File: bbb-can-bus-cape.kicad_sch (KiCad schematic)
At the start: 5 parts, among them P1 DG301-5.0-03P-12-00A(H), P2 DG301-5.0-03P-12-00A(H), P7 DG301-5.0-03P-12-00A(H), P8 BeagleBone_Black_Header, P9 BeagleBone_Black_Header

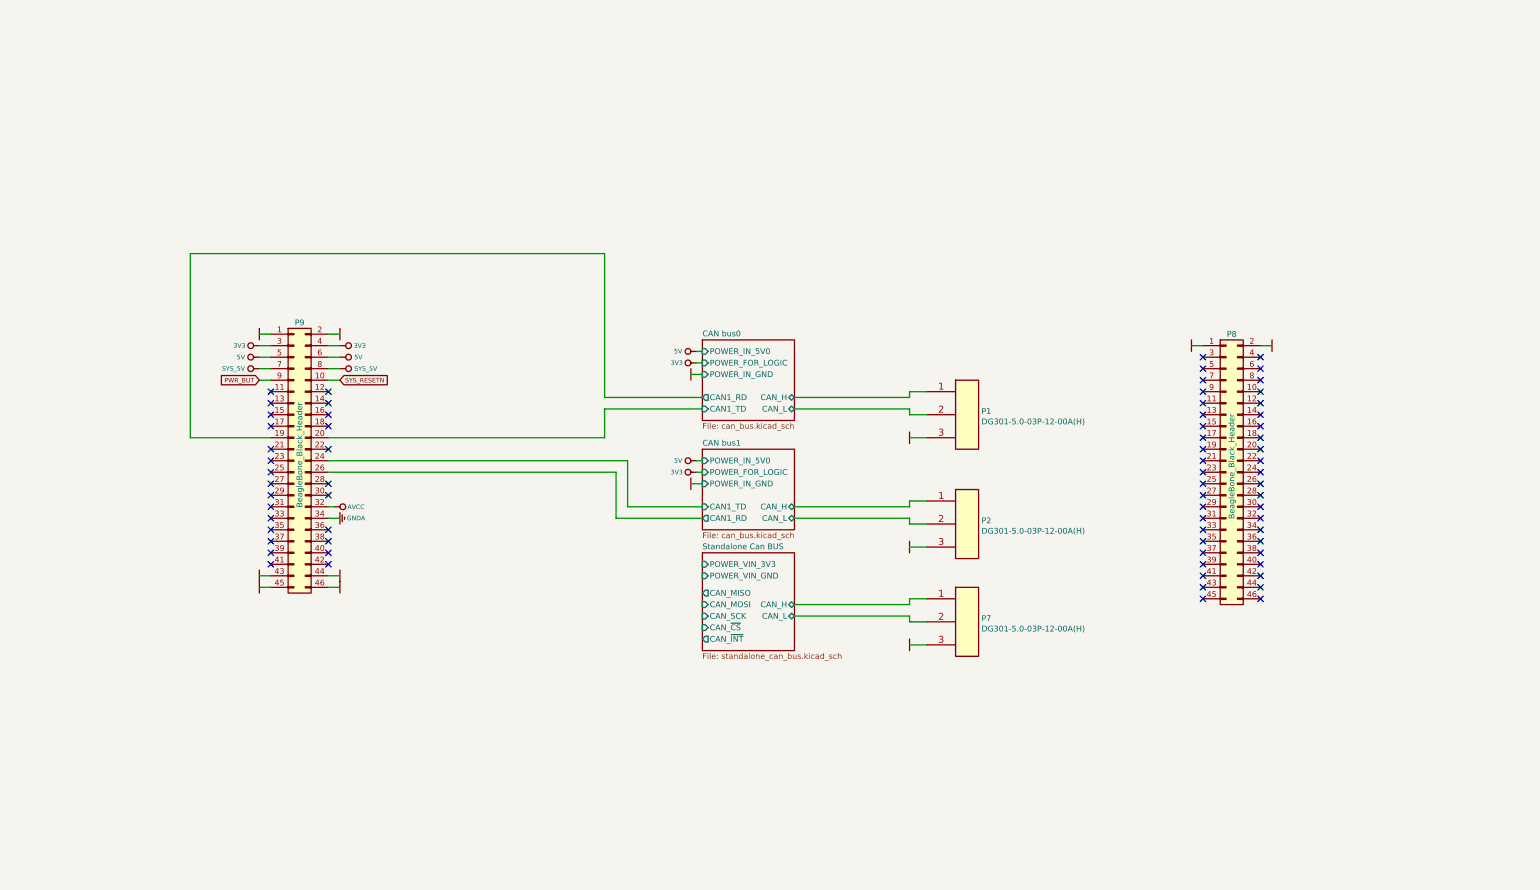
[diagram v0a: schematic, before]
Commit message: Schematic checked
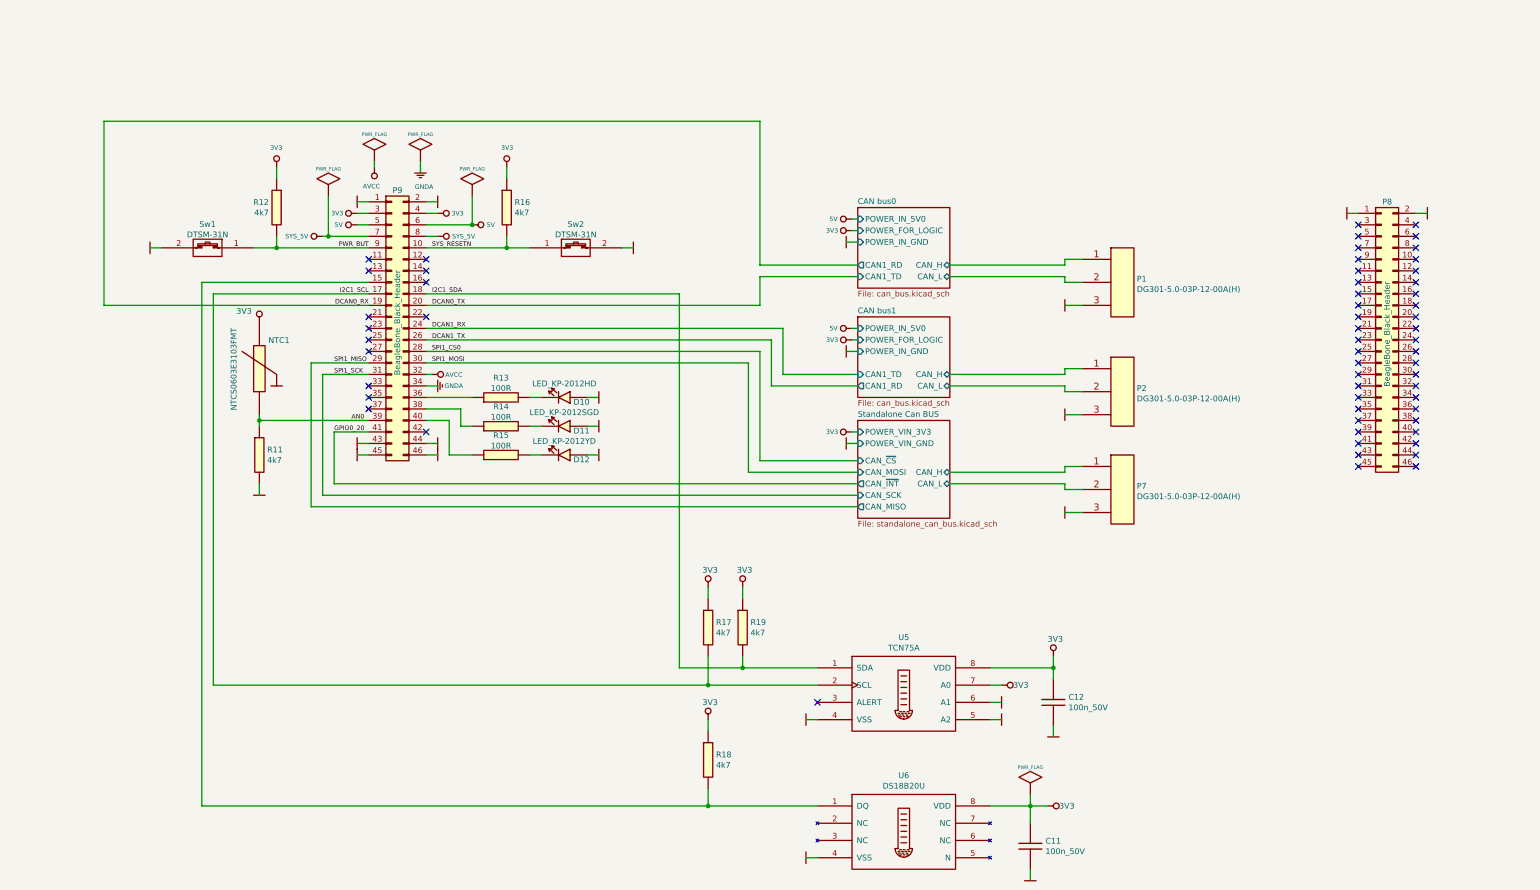
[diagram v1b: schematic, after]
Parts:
- added C11, C12: 100n_50V, Capacitors_Smd_0603:100nF_0603, symbol Capacitors_Smd0603:100n
- added D10: LED_KP-2012HD, Diodes:LED_KP-2012HD_SM0805, symbol Diodes:LED_KP-2012HD
- added D11: LED_KP-2012SGD, Diodes:LED_KP-2012SGD_SM0805, symbol Diodes:LED_KP-2012SGD
- added D12: LED_KP-2012YD, Diodes:LED_KP-2012YD_SM0805, symbol Diodes:LED_KP-2012YD
- added NTC1: NTCS0603E3103FMT, NTC_Thermistors:NTCS0603E3103FMT, symbol NTC_Thermistors:NTCS0603E3103FMT
- added R11, R12, R16, R17, R18, R19: 4k7, Resistor_Smd_0603:4k7_0603, symbol Resistors_Smd0603:4k7
- added R13, R14, R15: 100R, Resistor_Smd_0603:100R_0603, symbol Resistors_Smd0603:100R
- added Sw1, Sw2: DTSM-31N, Microswitches:DTSM-31N_SMD, symbol Microswitches:DTSM-31N
- added U5: TCN75A, Temperature_Sensors:TCN75A_SOIC8, symbol Temperature_Sensors:TCN75A
- added U6: DS18B20U, Temperature_Sensors:DS18B20U_MSOP-8_3x3mm_P0.65mm, symbol Temperature_Sensors:DS18B20U
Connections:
- net 3V3: now also C11.1, C12.1, NTC1.2, R12.1, R16.1, R17.1, R18.1, R19.1, U5.7 (A0), U5.8 (VDD), U6.8 (VDD)
- net GND: now also C11.2, C12.2, D10.1 (A), D11.1 (A), D12.1 (A), R11.2, Sw1.2, Sw2.2, U5.4 (VSS), U5.5 (A2), U5.6 (A1), U6.4 (VSS)
- net PWR_BUT: now also R12.2, Sw1.1
- net SYS_RESETN: now also R16.2, Sw2.1
- net at P9.15 (Pin_15): now also R18.2, U6.1 (DQ)
- net I2C1_SCL: now reaches P9.17 (Pin_17)
- net I2C1_SCL: now also R17.2, U5.2 (SCL)
- net I2C1_SDA: now reaches P9.18 (Pin_18)
- net I2C1_SDA: now also R19.2, U5.1 (SDA)
- net SPI1_CS0: now reaches P9.28 (Pin_28)
- net SPI1_MISO: now reaches P9.29 (Pin_29)
- net SPI1_MOSI: now reaches P9.30 (Pin_30)
- net SPI1_SCK: now reaches P9.31 (Pin_31)
- net at P9.36 (Pin_36): now also R13.1
- net at P9.38 (Pin_38): now also R14.1
- net AN0: now reaches P9.39 (Pin_39)
- net AN0: now also NTC1.1, R11.1
- net at P9.40 (Pin_40): now also R15.1
- net GPIO0_20: now reaches P9.41 (Pin_41)
- net CAN bus0/CAN1_RD renamed DCAN0_RX
- net CAN bus0/CAN1_TD renamed DCAN0_TX
- net CAN bus1/CAN1_RD renamed DCAN1_TX
- net CAN bus1/CAN1_TD renamed DCAN1_RX
- new net: D11.2 (K), R14.2
- new net: D10.2 (K), R13.2
- new net: D12.2 (K), R15.2
- no-connect marks 70 -> 59
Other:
- moved on the sheet: P1, P2, P7, P8, P9

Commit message: Finalized project
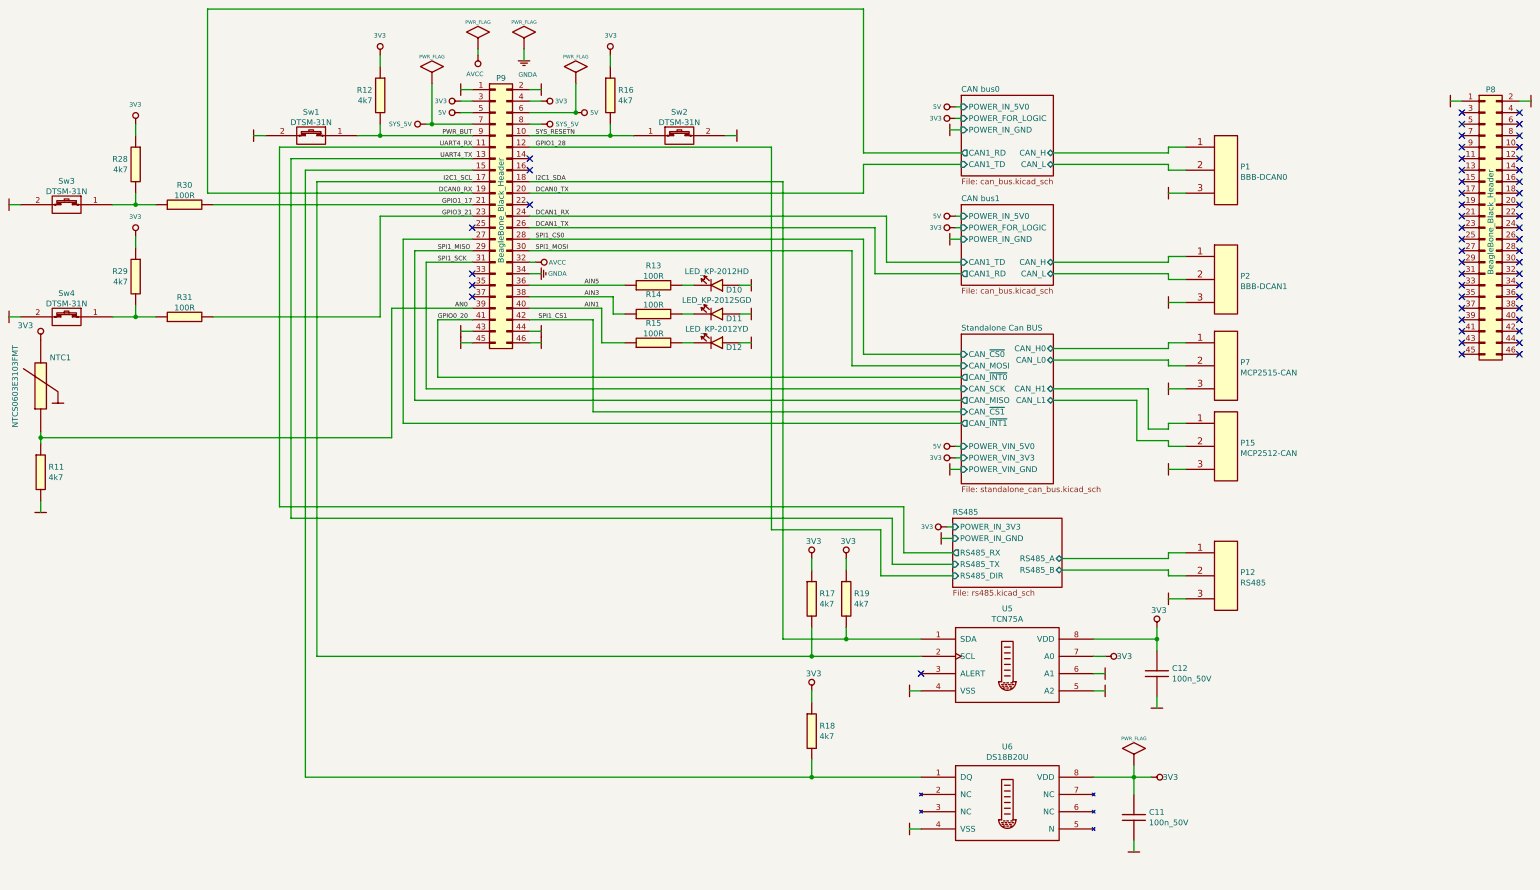
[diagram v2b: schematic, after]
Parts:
- added P12: RS485, Discrete_Connectors:DG301-5.0-03P-12-00A(H), symbol Discrete_Connectors:DG301-5.0-03P-12-00A(H)
- added P15: MCP2512-CAN, Discrete_Connectors:DG301-5.0-03P-12-00A(H), symbol Discrete_Connectors:DG301-5.0-03P-12-00A(H)
- added R28, R29: 4k7, Resistor_Smd_0603:4k7_0603, symbol Resistors_Smd0603:4k7
- added R30, R31: 100R, Resistor_Smd_0603:100R_0603, symbol Resistors_Smd0603:100R
- added Sw3, Sw4: DTSM-31N, Microswitches:DTSM-31N_SMD, symbol Microswitches:DTSM-31N
- P1: value DG301-5.0-03P-12-00A(H) -> BBB-DCAN0
- P2: value DG301-5.0-03P-12-00A(H) -> BBB-DCAN1
- P7: value DG301-5.0-03P-12-00A(H) -> MCP2515-CAN
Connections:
- net 3V3: now also R28.1, R29.1
- net GND: now also P12.3, P15.3, Sw3.2, Sw4.2
- net UART4_RX: now reaches P9.11 (Pin_11)
- net GPIO1_28: now reaches P9.12 (Pin_12)
- net UART4_TX: now reaches P9.13 (Pin_13)
- net GPIO1_17: now reaches P9.21 (Pin_21)
- net GPIO1_17: now also R30.2
- net GPIO3_21: now reaches P9.23 (Pin_23)
- net GPIO3_21: now also R31.2
- net Standalone Can BUS/CAN_~INT1~: now reaches P9.27 (Pin_27)
- net AIN5: now reaches P9.36 (Pin_36), R13.1
- net AIN3: now reaches P9.38 (Pin_38), R14.1
- net AIN1: now reaches P9.40 (Pin_40), R15.1
- net SPI1_CS1: now reaches P9.42 (Pin_42)
- net Standalone Can BUS/CAN_H renamed Standalone Can BUS/CAN_H0
- net Standalone Can BUS/CAN_L renamed Standalone Can BUS/CAN_L0
- new net: R29.2, R31.1, Sw4.1
- new net: R28.2, R30.1, Sw3.1
- new net RS485/RS485_A: P12.1
- new net RS485/RS485_B: P12.2
- new net Standalone Can BUS/CAN_H1: P15.1
- new net Standalone Can BUS/CAN_L1: P15.2
- no-connect marks 59 -> 52
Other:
- added sheet RS485 (rs485.kicad_sch)
- sheet Standalone Can BUS ports: added CAN_H0, CAN_H1, CAN_L0, CAN_L1, CAN_~CS0~, CAN_~CS1~, CAN_~INT0~, CAN_~INT1~, POWER_VIN_5V0; removed CAN_H, CAN_L, CAN_~CS~, CAN_~INT~
- moved on the sheet: C11, C12, D10, D11, D12, NTC1, P1, P2, P7, P8, P9, R11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
